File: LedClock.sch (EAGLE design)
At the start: 42 parts

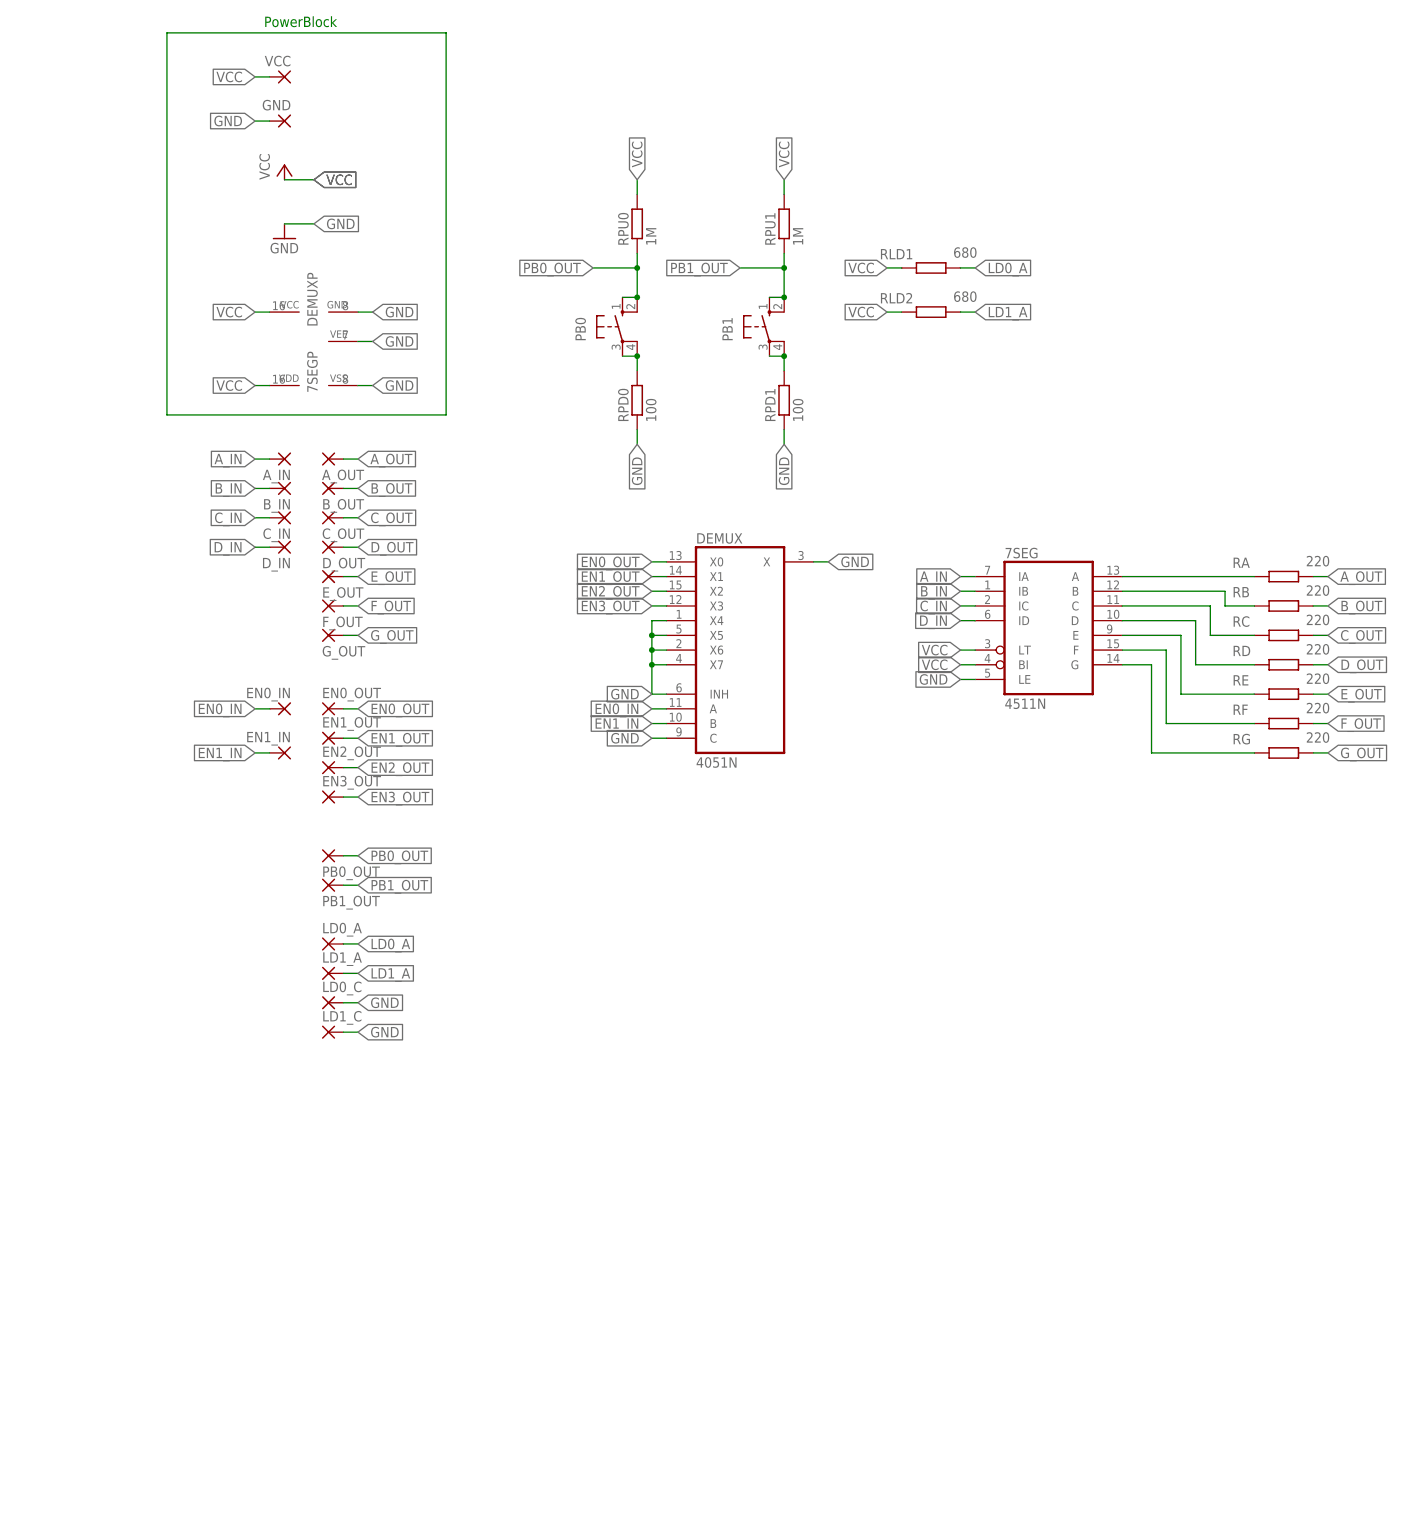
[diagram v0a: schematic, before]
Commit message: new sch, win10 reinstall
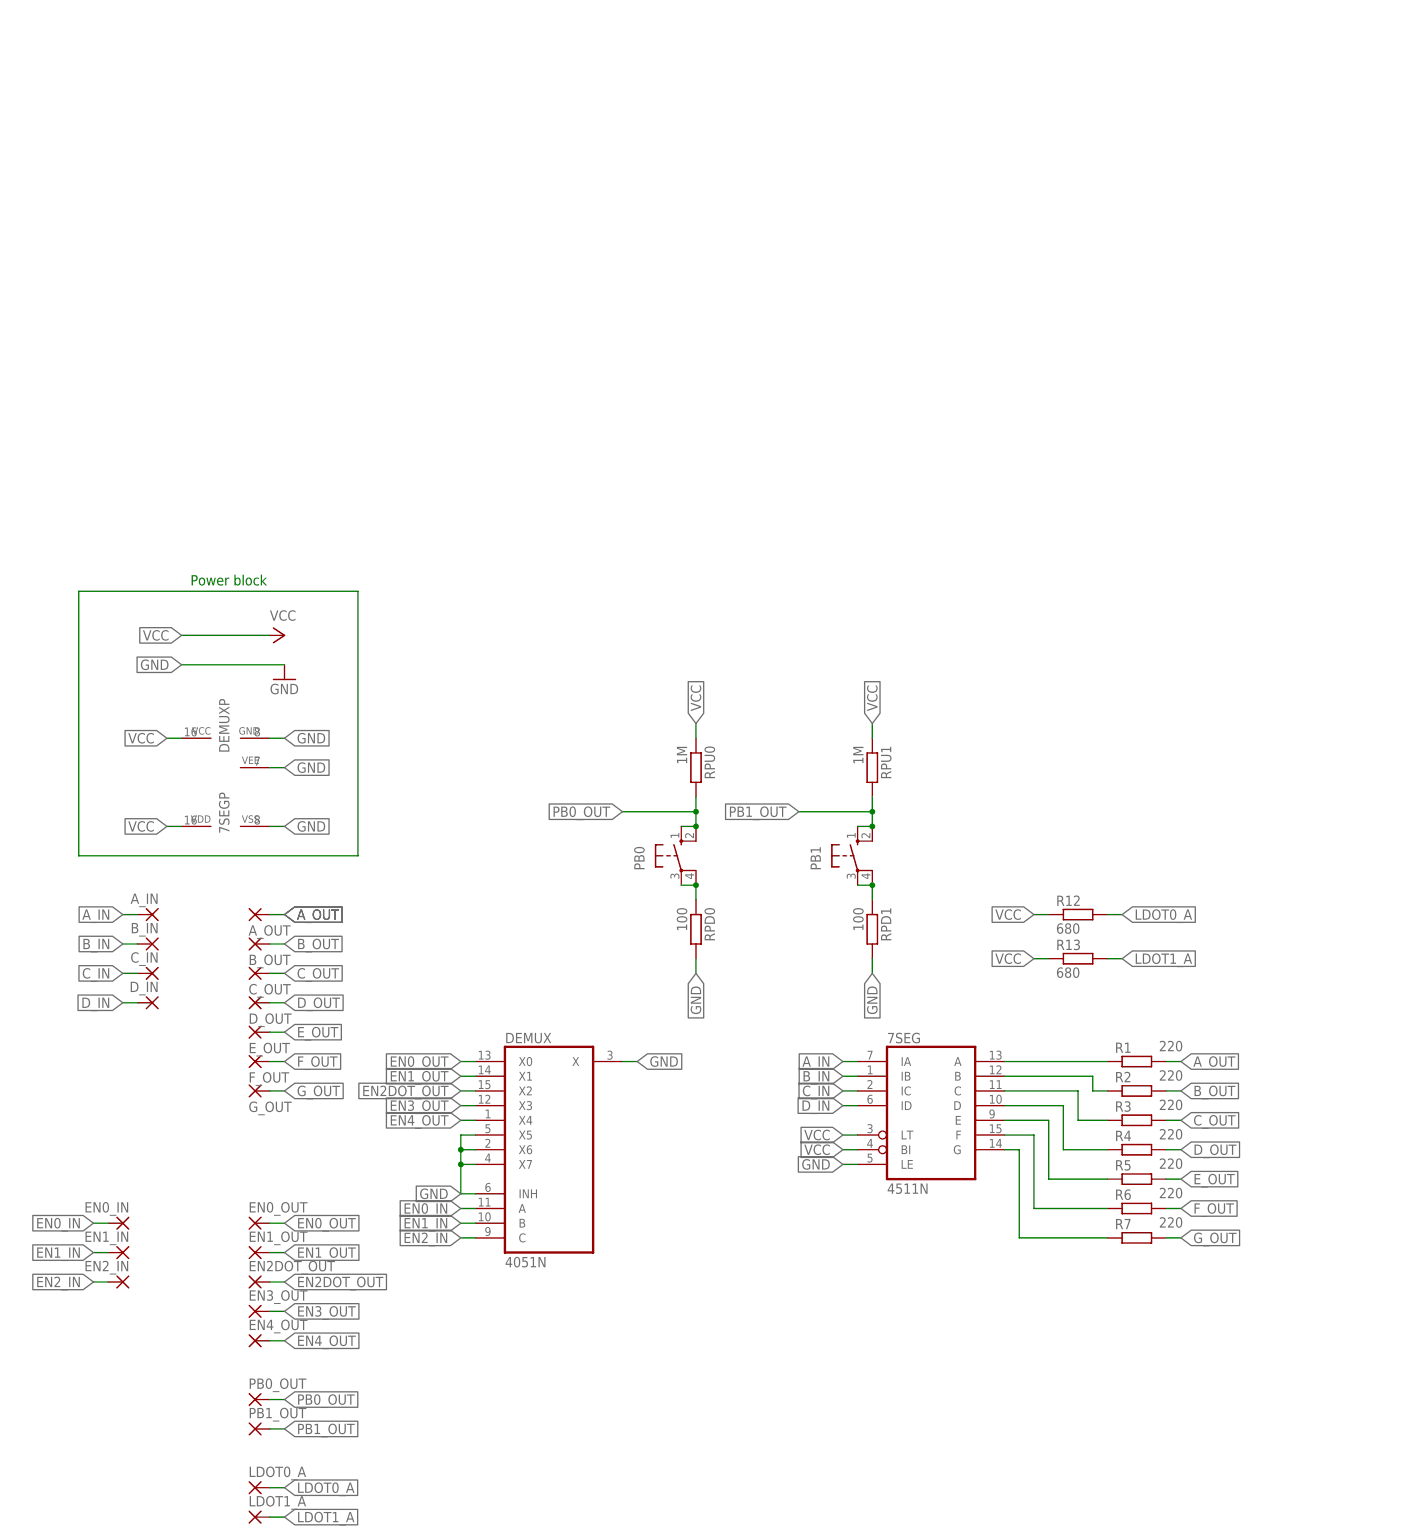
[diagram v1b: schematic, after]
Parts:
- removed EN2_OUT, GND, LD0_A, LD0_C, LD1_A, LD1_C, VCC: (no value), wirepad:2,54/1,0
- removed RA, RB, RC, RD, RE, RF, RG: 220, rcl:R-EU_R1206
- removed RLD1, RLD2: 680, rcl:R-EU_R1206
- added EN2DOT_OUT, EN2_IN, EN4_OUT, LDOT0_A, LDOT1_A: (no value), wirepad:2,54/1,0
- added R1, R2, R3, R4, R5, R6, R7: 220, rcl:R-EU_R1206
- added R12, R13: 680, rcl:R-EU_R1206
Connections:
- removed net EN2_OUT: DEMUXA.X2, EN2_OUT.P
- removed net LD0_A: LD0_A.P, RLD1.2
- removed net LD1_A: LD1_A.P, RLD2.2
- removed net N$10: 7SEGA.C, RC.1
- removed net N$11: 7SEGA.D, RD.1
- removed net N$12: 7SEGA.E, RE.1
- removed net N$13: 7SEGA.F, RF.1
- removed net N$14: 7SEGA.G, RG.1
- new net EN2DOT_OUT: DEMUXA.X2, EN2DOT_OUT.P
- new net EN2_IN: DEMUXA.C, EN2_IN.P
- new net EN4_OUT: DEMUXA.X4, EN4_OUT.P
- new net LDOT0_A: LDOT0_A.P, R12.2
- new net LDOT1_A: LDOT1_A.P, R13.2
- new net N$3: 7SEGA.C, R3.1
- new net N$4: 7SEGA.D, R4.1
- new net N$5: 7SEGA.E, R5.1
- new net N$6: 7SEGA.F, R6.1
- new net N$7: 7SEGA.G, R7.1
- net A_OUT: now also R1.2; no longer RA.2
- net B_OUT: now also R2.2; no longer RB.2
- net C_OUT: now also R3.2; no longer RC.2
- net D_OUT: now also R4.2; no longer RD.2
- net E_OUT: now also R5.2; no longer RE.2
- net F_OUT: now also R6.2; no longer RF.2
- net GND: now also RPD0.2, RPD1.2; no longer DEMUXA.C, DEMUXA.X4, GND.P, LD0_C.P, LD1_C.P, RPD0.1, RPD1.1
- net G_OUT: now also R7.2; no longer RG.2
- net N$1: now also 7SEGA.A, R1.1; no longer PB1.P, PB1.P1, RPD1.2
- net N$2: now also 7SEGA.B, R2.1; no longer PB0.P, PB0.P1, RPD0.2
- net N$8: now also PB0.P, PB0.P1, RPD0.1; no longer 7SEGA.A, RA.1
- net N$9: now also PB1.P, PB1.P1, RPD1.1; no longer 7SEGA.B, RB.1
- net PB0_OUT: now also RPU0.2; no longer RPU0.1
- net PB1_OUT: now also RPU1.2; no longer RPU1.1
- net VCC: now also R12.1, R13.1, RPU0.1, RPU1.1; no longer RLD1.1, RLD2.1, RPU0.2, RPU1.2, VCC.P
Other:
- note added: "Power block"
- note removed: "PowerBlock"
- moved on the sheet: 7SEG, 7SEGP, A_IN, A_OUT, B_IN, B_OUT, C_IN, C_OUT, DEMUX, DEMUXP, D_IN, D_OUT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
